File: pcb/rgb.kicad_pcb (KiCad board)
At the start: 2 copper layers, 128 x 30 mm, 16 parts, among them J1 Conn_02x08_Odd_Even, J2 Conn_01x06, J3 Conn_01x02, U1 ESP-WROOM-32, U2 LM317EMP, U3 RASPI_SD

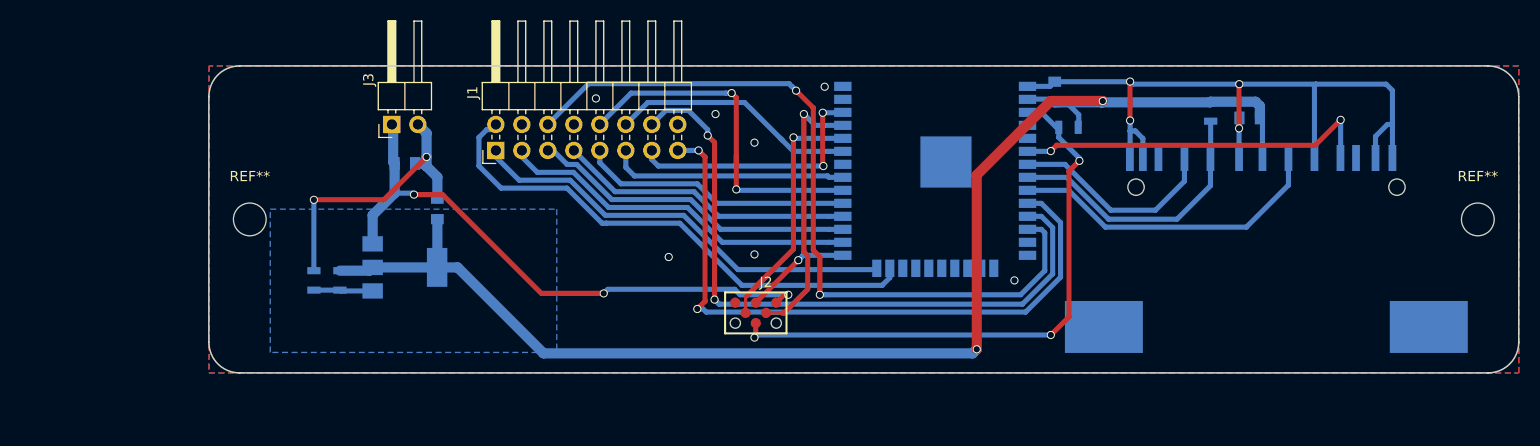
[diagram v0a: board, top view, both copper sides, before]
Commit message: PCB REV1
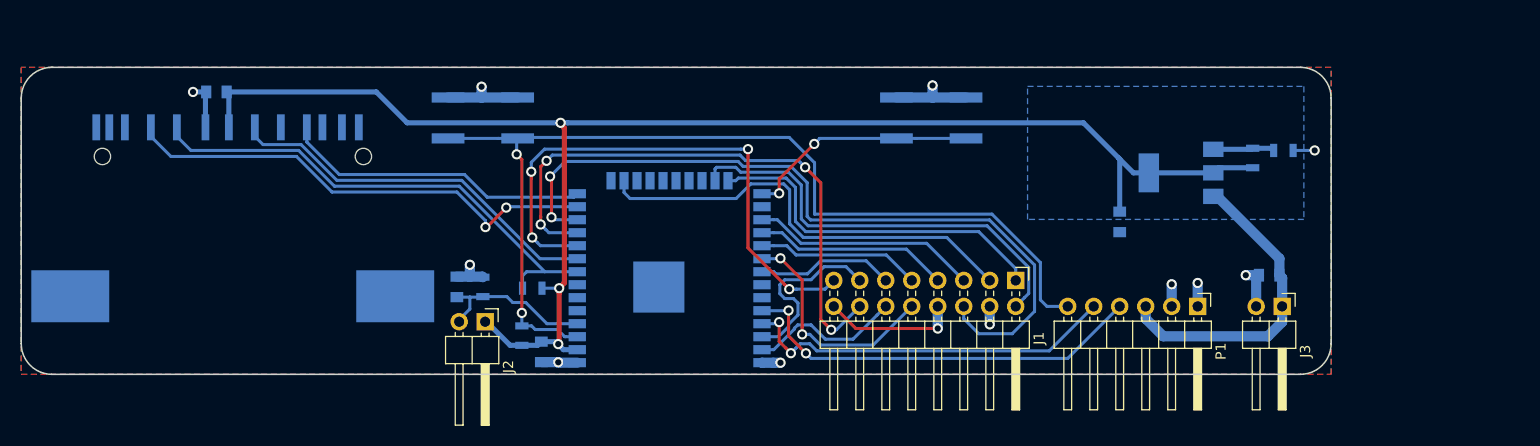
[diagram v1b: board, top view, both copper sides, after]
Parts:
- removed REF** (x2): MountingHole_3.2mm_M3, Mounting_Holes:MountingHole_3.2mm_M3
- added C5: 1u, Capacitors_SMD:C_0805, B.Cu at (102.2, 61.6)
- added P1: TTL_232R_3V3, Pin_Headers:Pin_Header_Angled_1x06_Pitch2.54mm, F.Cu at (174.6, 63.5)
- added R6: 10k, Resistors_SMD:R_0805, B.Cu at (104.8, 61.6)
- added U4: TACTILE, myStuff:EVQQ2, B.Cu at (104.8, 45.1)
- added U5: TACTILE, myStuff:EVQQ2, B.Cu at (148.6, 45.1)
- J2: value Conn_01x06 -> Conn_01x02; footprint myStuff:myPogoPads -> Pin_Headers:Pin_Header_Angled_1x02_Pitch2.54mm
- moved U3 101.0 mm to (67.0, 46.0)
- moved C4 101.0 mm to (78.7, 42.5), turned to 180 degrees
- moved R3 95.6 mm to (183.0, 48.3), turned to 0 degrees
- moved R2 90.0 mm to (180.0, 49.0), turned to 90 degrees
- moved J3 88.8 mm to (182.9, 63.5), turned to 270 degrees
- moved C3 85.2 mm to (181.6, 60.5), turned to 0 degrees
- moved U2 76.4 mm to (173.0, 50.5), turned to 180 degrees
- moved R4 68.5 mm to (109.6, 61.7), turned to 0 degrees
- moved C2 66.7 mm to (167.0, 55.2), turned to 90 degrees
- moved R1 57.2 mm to (108.6, 66.4), turned to 90 degrees
- moved C1 56.2 mm to (110.5, 67.9), turned to 90 degrees
- moved J1 52.4 mm to (156.8, 61.0), turned to 270 degrees
- moved U1 51.6 mm to (114.0, 69.0), turned to 0 degrees
- moved J2 26.5 mm to (105.0, 65.0), turned to 270 degrees
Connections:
- C4 pad 1: GND -> +3V3
- C4 pad 2: +3V3 -> GND
- J2 pad 1: /rstBtn -> +3V3
- J2 pad 2: Net-(J2-Pad2) -> Net-(C5-Pad1)
- U1 pad 13: Net-(U1-Pad13) -> /SD_CS
- U1 pad 14: Net-(U1-Pad14) -> /SD_MISO
- U1 pad 16: Net-(U1-Pad16) -> /B0
- U1 pad 26: /B0 -> Net-(U1-Pad26)
- U1 pad 33: /D -> Net-(U1-Pad33)
- U1 pad 34: Net-(J2-Pad3) -> Net-(P1-Pad4)
- U1 pad 35: Net-(J2-Pad2) -> Net-(P1-Pad5)
- U1 pad 37: Net-(U1-Pad37) -> /D
- U1 pad 4: Net-(U1-Pad4) -> Net-(C5-Pad1)
- U1 pad 6: /SD_MISO -> Net-(U1-Pad6)
- U1 pad 7: /SD_CS -> Net-(U1-Pad7)
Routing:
- net GND: track 102.5 -> 55.6 mm, vias 13 -> 12
- net Net-(P1-Pad4): track 0.00 -> 40.5 mm, vias 0 -> 2
- net /rstBtn: track 56.5 -> 96.9 mm, vias 3 -> 2
- net Net-(P1-Pad5): track 0.00 -> 37.3 mm, vias 0 -> 2
- net /SD_CS: track 20.6 -> 47.4 mm, vias 0 -> 2
- net Net-(J2-Pad2): track 26.6 -> 0.00 mm, vias 1 -> 0
- net Net-(J2-Pad3): track 26.2 -> 0.00 mm, vias 1 -> 0
- net +5V: track 57.1 -> 31.1 mm, vias 3 -> 0
- net /SD_MOSI: track 28.1 -> 49.0 mm
- net Net-(C5-Pad1): track 0.00 -> 15.7 mm
- net /B: track 37.5 -> 22.8 mm
- net /progFlag: track 10.4 -> 23.0 mm, vias 1 -> 2
- net +3V3: track 135.6 -> 147.0 mm, vias 2 -> 3
- net /OE: track 64.5 -> 53.9 mm, vias 2 -> 4
- net /A: track 26.6 -> 16.0 mm
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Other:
- net class Default: via_dia 0.8 -> 1
